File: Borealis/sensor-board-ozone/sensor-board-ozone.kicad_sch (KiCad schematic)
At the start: 7 parts, among them J1 Conn_01x02_Pin (Solar panel c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, J2 Conn_01x03_Pin (data connecti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, J5 Conn_01x03_Pin (power connect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

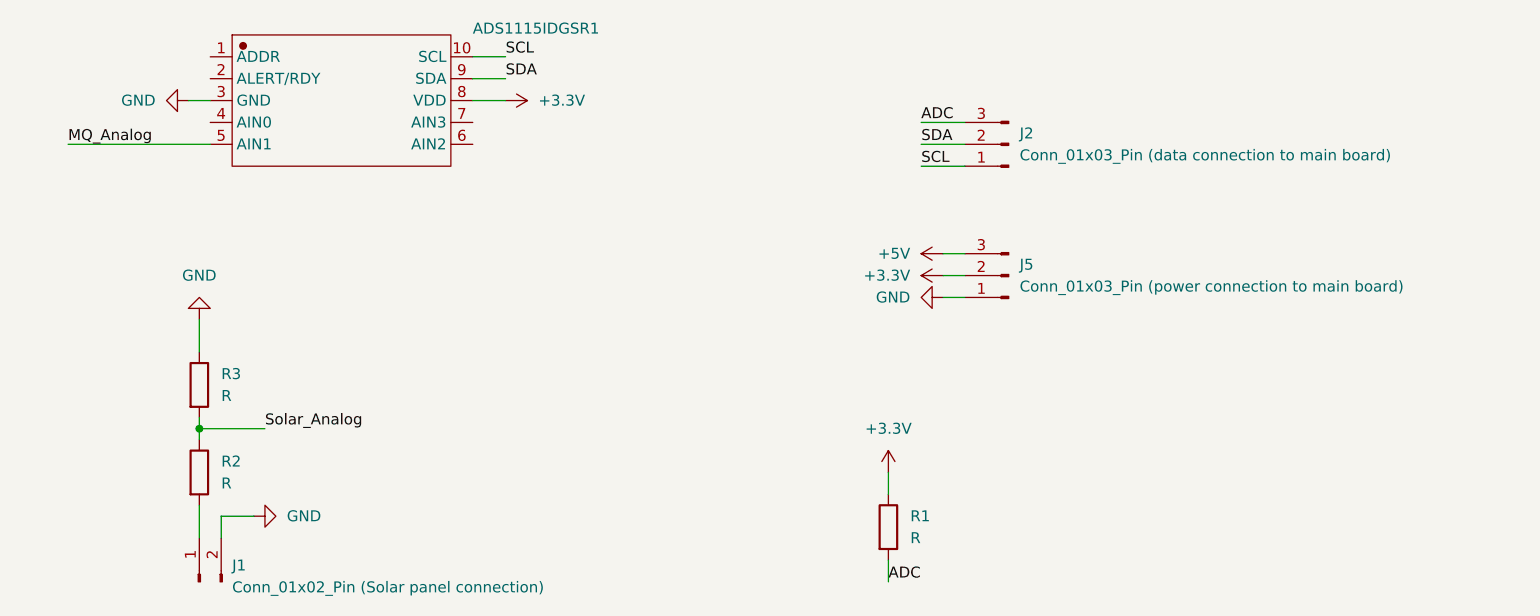
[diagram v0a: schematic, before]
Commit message: Fixed a few things
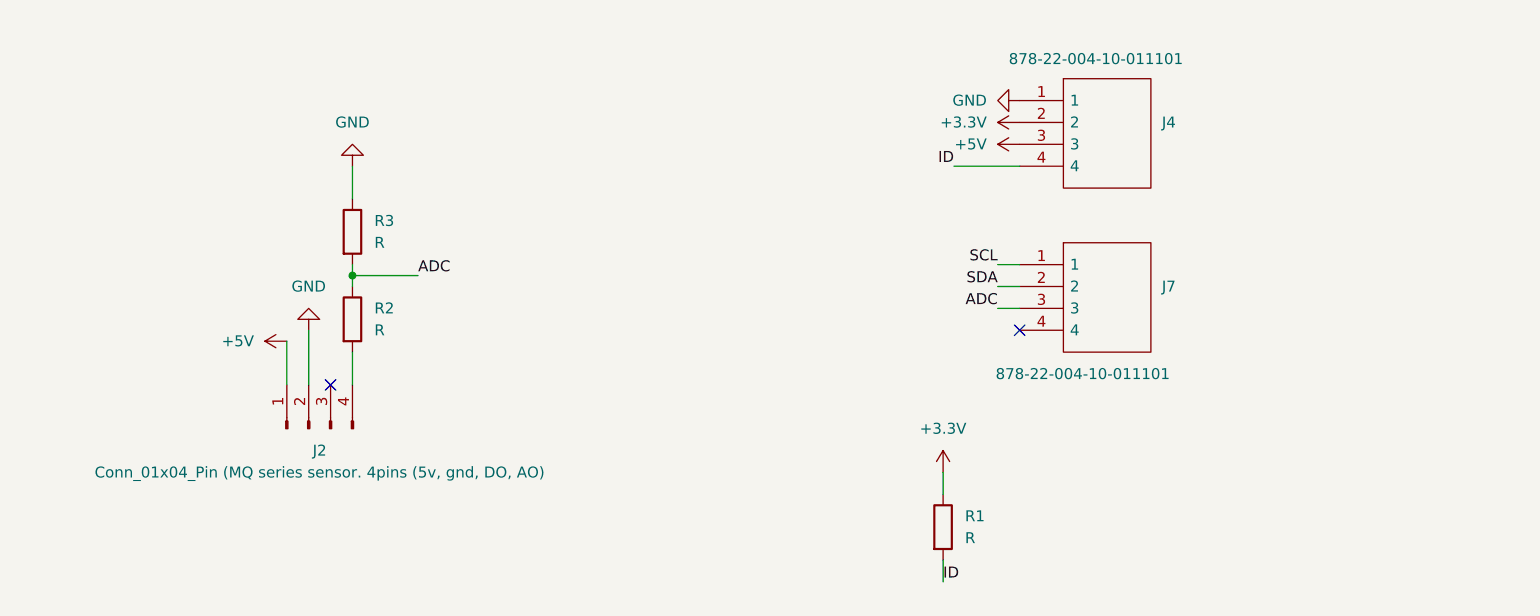
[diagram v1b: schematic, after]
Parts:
- removed ADS1115IDGSR1: ~, batteryholder:ADS1115IDGSR, symbol ADS1115IDGSR_2025-12-25-altium-import:root_0_ADS1115IDGSR_
- removed J1: Conn_01x02_Pin (Solar panel connection), symbol Connector:Conn_01x02_Pin
- removed J2: Conn_01x03_Pin (data connection to main board), symbol Connector:Conn_01x03_Pin
- removed J5: Conn_01x03_Pin (power connection to main board), symbol Connector:Conn_01x03_Pin
- added J2: Conn_01x04_Pin (MQ series sensor. 4pins (5v, gnd,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, symbol Connector:Conn_01x04_Pin
- added J4, J7: 878-22-004-10-011101, BOREALIS:8782200410011101, symbol 878-22-004-10-011101:878-22-004-10-011101
- R1: footprint OptoDevice:R_LDR_4.9x4.2mm_P2.54mm_Vertical -> Resistor_SMD:R_0805_2012Metric
- R2, R3: footprint (none) -> Resistor_SMD:R_0805_2012Metric
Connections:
- net Solar_Analog is gone; now on net ADC: R2.1, R3.2
- net +3.3V: now also J4.2
- net +5V: now also J2.1 (Pin_1), J4.3
- net ADC: now also J7.3; no longer R1.2
- net GND: now also J2.2 (Pin_2), J4.1
- net SCL: now also J7.1
- net SDA: now also J7.2
- net at R2.2: now also J2.4 (Pin_4)
- new net ID: J4.4, R1.2
- no-connect marks 0 -> 2
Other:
- moved on the sheet: R1, R2, R3
